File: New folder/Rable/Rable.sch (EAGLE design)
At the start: 199 parts, among them J1 TYPE-C-31-M-12, J3 I2C-HEADER, J4 I2C-HEADER, J5 I2C-HEADER, U1 HOLYIOT-18010-NRF52840, U2 AP2112K-3.3TRG1, U3 LTC4054, U4 AO3401, U5 AO3401, X1 SM04B-SRSS-TB, X2 BM06B-SRSS-TB, X3 BM06B-SRSS-TB, X4 BM06B-SRSS-TB

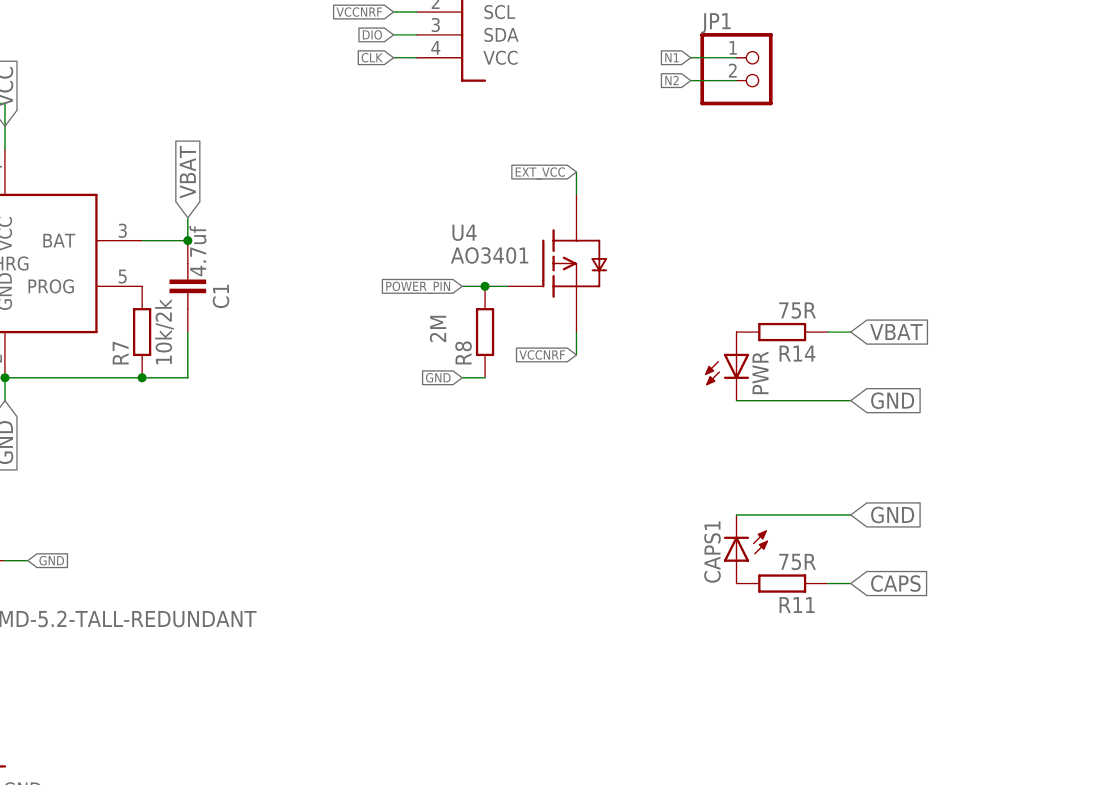
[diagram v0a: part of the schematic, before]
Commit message: add
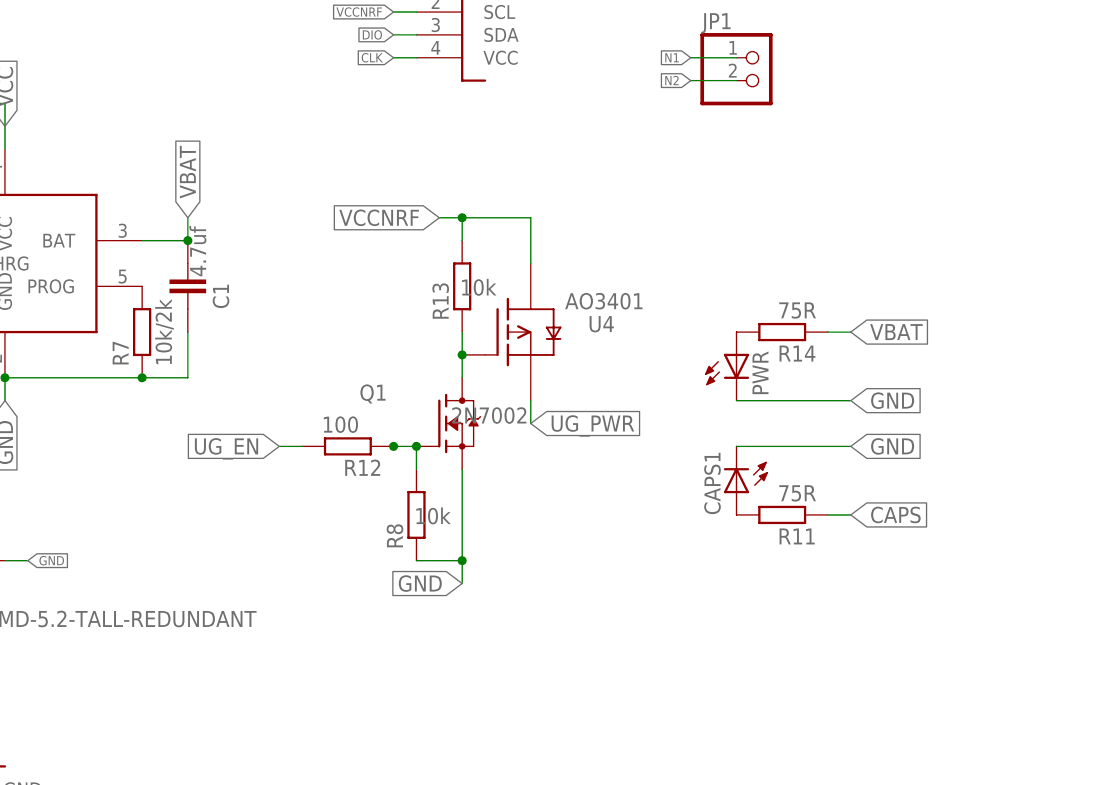
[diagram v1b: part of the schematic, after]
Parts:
- added Q1: 2N7002, 2N7002:2N7002
- added R12: 100, Components:RESISTOR-0805
- added R13: 10k, Components:RESISTOR-0805
- R8: value 2M -> 10k
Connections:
- new net N$51: Q1.G, R12.1, R8.2
- new net N$53: Q1.D, R13.1, U4.G
- new net UG_EN: R12.2
- new net UG_PWR: U4.S
- net EXT_VCC: no longer U4.D
- net GND: now also Q1.S
- net POWER_PIN: no longer R8.2, U4.G
- net VCCNRF: now also R13.2, U4.D; no longer U4.S
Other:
- moved on the sheet: CAPS1, R11, R8, U4
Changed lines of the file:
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@@
 <part name="E1" library="SRV05-4.TCT" deviceset="SRV05-4.TCT" device=""/>
 <part name="U4" library="AO3401" deviceset="AO3401" device=""/>
-<part name="R8" library="Components" deviceset="RESISTOR" device="-0805" value="2M"/>
+<part name="R8" library="Components" deviceset="RESISTOR" device="-0805" value="10k"/>
 <part name="J3" library="Headers" deviceset="I2C-HEADER" device=""/>
 <part name="R11" library="Components" deviceset="RESISTOR" device="-0805" value="75R"/>
@@
 <part name="BAT2" library="adafruit" deviceset="JST_2PIN" device="-THM-RA"/>
 <part name="LED1" library="adafruit" deviceset="LED" device="CHIPLED_1206"/>
+<part name="Q1" library="2N7002" deviceset="2N7002" device=""/>
+<part name="R12" library="Components" deviceset="RESISTOR" device="-0805" value="100"/>
+<part name="R13" library="Components" deviceset="RESISTOR" device="-0805" value="10k"/>
 </parts>
 <sheets>
@@
 <attribute name="VALUE" x="-219.71" y="119.38" size="1.778" layer="96" align="center-left"/>
 </instance>
-<instance part="U4" gate="G$1" x="-137.16" y="63.5" smashed="yes">
-<attribute name="VALUE" x="-148.59" y="63.5" size="1.778" layer="96"/>
-<attribute name="NAME" x="-148.59" y="66.04" size="1.778" layer="95"/>
-</instance>
-<instance part="R8" gate="G$1" x="-144.78" y="55.88" smashed="yes" rot="R90">
-<attribute name="NAME" x="-146.2786" y="52.07" size="1.778" layer="95" rot="R90"/>
-<attribute name="VALUE" x="-149.098" y="54.61" size="1.778" layer="96" rot="R90"/>
+<instance part="U4" gate="G$1" x="-142.24" y="55.88" smashed="yes">
+<attribute name="VALUE" x="-135.89" y="58.42" size="1.778" layer="96"/>
+<attribute name="NAME" x="-133.35" y="55.88" size="1.778" layer="95"/>
+</instance>
+<instance part="R8" gate="G$1" x="-152.4" y="35.56" smashed="yes" rot="R90">
+<attribute name="NAME" x="-153.8986" y="31.75" size="1.778" layer="95" rot="R90"/>
+<attribute name="VALUE" x="-148.59" y="36.322" size="1.778" layer="96" rot="R180"/>
 </instance>
 <instance part="J3" gate="G$1" x="-149.86" y="91.44" smashed="yes" rot="R180"/>
-<instance part="R11" gate="G$1" x="-111.76" y="27.94" smashed="yes" rot="R180">
-<attribute name="NAME" x="-107.95" y="26.4414" size="1.778" layer="95" rot="R180"/>
-<attribute name="VALUE" x="-107.95" y="31.242" size="1.778" layer="96" rot="R180"/>
+<instance part="R11" gate="G$1" x="-111.76" y="35.56" smashed="yes" rot="R180">
+<attribute name="NAME" x="-107.95" y="34.0614" size="1.778" layer="95" rot="R180"/>
+<attribute name="VALUE" x="-107.95" y="38.862" size="1.778" layer="96" rot="R180"/>
 </instance>
 <instance part="JP1" gate="G$1" x="-114.3" y="83.82" smashed="yes">
@@
 <attribute name="VALUE" x="-111.125" y="48.768" size="1.778" layer="96" rot="R90"/>
 </instance>
-<instance part="CAPS1" gate="G$1" x="-116.84" y="30.48" smashed="yes" rot="R180">
-<attribute name="NAME" x="-120.396" y="35.052" size="1.778" layer="95" rot="R270"/>
-<attribute name="VALUE" x="-122.555" y="35.052" size="1.778" layer="96" rot="R270"/>
+<instance part="CAPS1" gate="G$1" x="-116.84" y="38.1" smashed="yes" rot="R180">
+<attribute name="NAME" x="-120.396" y="42.672" size="1.778" layer="95" rot="R270"/>
+<attribute name="VALUE" x="-122.555" y="42.672" size="1.778" layer="96" rot="R270"/>
 </instance>
 <instance part="RGB1" gate="G$1" x="-281.94" y="165.1" smashed="yes">
@@
 <attribute name="NAME" x="-204.724" y="66.548" size="1.778" layer="95" rot="R90"/>
 <attribute name="VALUE" x="-202.565" y="64.008" size="1.778" layer="96" rot="R90"/>
+</instance>
+<instance part="Q1" gate="G$1" x="-149.86" y="45.72" smashed="yes">
+<attribute name="VALUE" x="-148.59" y="45.72" size="1.778" layer="96"/>
+<attribute name="NAME" x="-158.75" y="48.26" size="1.778" layer="95"/>
+</instance>
+<instance part="R12" gate="G$1" x="-160.02" y="43.18" smashed="yes" rot="R180">
+<attribute name="NAME" x="-156.21" y="41.6814" size="1.778" layer="95" rot="R180"/>
+<attribute name="VALUE" x="-158.75" y="46.482" size="1.778" layer="96" rot="R180"/>
+</instance>
+<instance part="R13" gate="G$1" x="-147.32" y="60.96" smashed="yes" rot="R90">
+<attribute name="NAME" x="-148.8186" y="57.15" size="1.778" layer="95" rot="R90"/>
+<attribute name="VALUE" x="-143.51" y="61.722" size="1.778" layer="96" rot="R180"/>
 </instance>
 </instances>
@@
 </segment>
 <segment>
-<pinref part="R8" gate="G$1" pin="1"/>
-<wire x1="-144.78" y1="50.8" x2="-147.32" y2="50.8" width="0.1524" layer="91"/>
-<label x="-147.32" y="50.8" size="1.016" layer="95" rot="R180" xref="yes"/>
-</segment>
-<segment>
 <pinref part="U1" gate="G$1" pin="GND"/>
 <wire x1="-248.92" y1="-53.34" x2="-246.38" y2="-53.34" width="0.1524" layer="91"/>
@@
 </segment>
 <segment>
-<label x="-104.14" y="35.56" size="1.778" layer="95" xref="yes"/>
+<label x="-104.14" y="43.18" size="1.778" layer="95" xref="yes"/>
 <pinref part="CAPS1" gate="G$1" pin="C"/>
-<wire x1="-116.84" y1="35.56" x2="-104.14" y2="35.56" width="0.1524" layer="91"/>
+<wire x1="-116.84" y1="43.18" x2="-104.14" y2="43.18" width="0.1524" layer="91"/>
 </segment>
 <segment>
@@
 <wire x1="-101.6" y1="116.84" x2="-88.9" y2="116.84" width="0.1524" layer="91"/>
 </segment>
+<segment>
+<pinref part="R8" gate="G$1" pin="1"/>
+<pinref part="Q1" gate="G$1" pin="S"/>
+<wire x1="-152.4" y1="30.48" x2="-147.32" y2="30.48" width="0.1524" layer="91"/>
+<wire x1="-147.32" y1="30.48" x2="-147.32" y2="40.64" width="0.1524" layer="91"/>
+<wire x1="-147.32" y1="30.48" x2="-147.32" y2="27.94" width="0.1524" layer="91"/>
+<junction x="-147.32" y="30.48"/>
+<label x="-147.32" y="27.94" size="1.778" layer="95" rot="R180" xref="yes"/>
+</segment>
 </net>
 <net name="VCC" class="0">
@@
 </segment>
 <segment>
-<pinref part="U4" gate="G$1" pin="S"/>
-<wire x1="-134.62" y1="55.88" x2="-134.62" y2="53.34" width="0.1524" layer="91"/>
-<label x="-134.62" y="53.34" size="1.016" layer="95" rot="R180" xref="yes"/>
-</segment>
-<segment>
 <pinref part="J5" gate="G$1" pin="SCL"/>
 <wire x1="-205.74" y1="2.54" x2="-215.9" y2="2.54" width="0.1524" layer="91"/>
@@
 <wire x1="-152.4" y1="91.44" x2="-154.94" y2="91.44" width="0.1524" layer="91"/>
 <label x="-154.94" y="91.44" size="1.016" layer="95" rot="R180" xref="yes"/>
+</segment>
+<segment>
+<pinref part="R13" gate="G$1" pin="2"/>
+<wire x1="-147.32" y1="66.04" x2="-147.32" y2="68.58" width="0.1524" layer="91"/>
+<pinref part="U4" gate="G$1" pin="D"/>
+<wire x1="-147.32" y1="68.58" x2="-139.7" y2="68.58" width="0.1524" layer="91"/>
+<wire x1="-139.7" y1="68.58" x2="-139.7" y2="63.5" width="0.1524" layer="91"/>
+<wire x1="-147.32" y1="68.58" x2="-149.86" y2="68.58" width="0.1524" layer="91"/>
+<junction x="-147.32" y="68.58"/>
+<label x="-149.86" y="68.58" size="1.778" layer="95" rot="R180" xref="yes"/>
 </segment>
 </net>
@@
 <net name="POWER_PIN" class="0">
 <segment>
-<pinref part="U4" gate="G$1" pin="G"/>
-<wire x1="-142.24" y1="60.96" x2="-144.78" y2="60.96" width="0.1524" layer="91"/>
-<pinref part="R8" gate="G$1" pin="2"/>
-<wire x1="-144.78" y1="60.96" x2="-147.32" y2="60.96" width="0.1524" layer="91"/>
-<junction x="-144.78" y="60.96"/>
-<label x="-147.32" y="60.96" size="1.016" layer="95" rot="R180" xref="yes"/>
-</segment>
-<segment>
 <pinref part="U1" gate="G$1" pin="P0.05"/>
 <wire x1="-294.64" y1="15.24" x2="-297.18" y2="15.24" width="0.1524" layer="91"/>
@@
 </net>
 <net name="EXT_VCC" class="0">
-<segment>
-<pinref part="U4" gate="G$1" pin="D"/>
-<wire x1="-134.62" y1="71.12" x2="-134.62" y2="73.66" width="0.1524" layer="91"/>
-<label x="-134.62" y="73.66" size="1.016" layer="95" rot="R180" xref="yes"/>
-</segment>
 <segment>
 <pinref part="RGB1" gate="G$1" pin="VDD"/>
@@
 <segment>
 <pinref part="R11" gate="G$1" pin="1"/>
-<wire x1="-106.68" y1="27.94" x2="-104.14" y2="27.94" width="0.1524" layer="91"/>
-<label x="-104.14" y="27.94" size="1.778" layer="95" xref="yes"/>
+<wire x1="-106.68" y1="35.56" x2="-104.14" y2="35.56" width="0.1524" layer="91"/>
+<label x="-104.14" y="35.56" size="1.778" layer="95" xref="yes"/>
 </segment>
 <segment>
@@
 </segment>
 </net>
+<net name="UG_EN" class="0">
+<segment>
+<pinref part="R12" gate="G$1" pin="2"/>
+<wire x1="-165.1" y1="43.18" x2="-167.64" y2="43.18" width="0.1524" layer="91"/>
+<label x="-167.64" y="43.18" size="1.778" layer="95" rot="R180" xref="yes"/>
+</segment>
+</net>
+<net name="N$53" class="0">
+<segment>
+<pinref part="R13" gate="G$1" pin="1"/>
+<pinref part="Q1" gate="G$1" pin="D"/>
+<wire x1="-147.32" y1="55.88" x2="-147.32" y2="53.34" width="0.1524" layer="91"/>
+<pinref part="U4" gate="G$1" pin="G"/>
+<wire x1="-147.32" y1="53.34" x2="-147.32" y2="50.8" width="0.1524" layer="91"/>
+<junction x="-147.32" y="53.34"/>
+</segment>
+</net>
+<net name="UG_PWR" class="0">
+<segment>
+<pinref part="U4" gate="G$1" pin="S"/>
+<wire x1="-139.7" y1="48.26" x2="-139.7" y2="45.72" width="0.1524" layer="91"/>
+<label x="-139.7" y="45.72" size="1.778" layer="95" xref="yes"/>
+</segment>
+</net>
+<net name="N$51" class="0">
+<segment>
+<pinref part="R12" gate="G$1" pin="1"/>
+<pinref part="R12" gate="G$1" pin="1"/>
+<pinref part="Q1" gate="G$1" pin="G"/>
+<wire x1="-154.94" y1="43.18" x2="-152.4" y2="43.18" width="0.1524" layer="91"/>
+<junction x="-154.94" y="43.18"/>
+<pinref part="R8" gate="G$1" pin="2"/>
+<wire x1="-152.4" y1="43.18" x2="-152.4" y2="40.64" width="0.1524" layer="91"/>
+<junction x="-152.4" y="43.18"/>
+</segment>
+</net>
